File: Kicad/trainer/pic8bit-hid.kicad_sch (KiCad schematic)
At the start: 27 parts, among them K402 SYMBOL-HEADER-F-1X10, K409 HARWIN-254-F-1X16-VERTICAL, K410 LED, P401 AN1, P402 AN2

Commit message: Update
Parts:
- S403: footprint tronixio:BOURNS-PEC12R -> tronixio:BOURNS-PEC12R-SWITCH; symbol tronixio:BOURNS-PEC12R-24DENTS -> tronixio:BOURNS-PEC12R-24DENTS-SWITCH-15MM
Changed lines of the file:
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@@
     (pin "1")
   )
-  (symbol (lib_id "tronixio:BOURNS-PEC12R-24DENTS") (at 104.14 96.52 0) (unit 1)
+  (symbol (lib_id "tronixio:BOURNS-PEC12R-24DENTS-SWITCH-15MM") (at 104.14 96.52 0) (unit 1)
     (in_bom yes) (on_board yes)
     (property "Reference" "S403" (id 0) (at 104.14 87.63 0)
@@
       (effects (font (size 1.15 1.15)) hide)
     )
-    (property "Footprint" "tronixio:BOURNS-PEC12R" (id 2) (at 104.14 111.76 0)
+    (property "Footprint" "tronixio:BOURNS-PEC12R-SWITCH" (id 2) (at 104.14 111.76 0)
       (effects (font (size 1 1)) hide)
     )

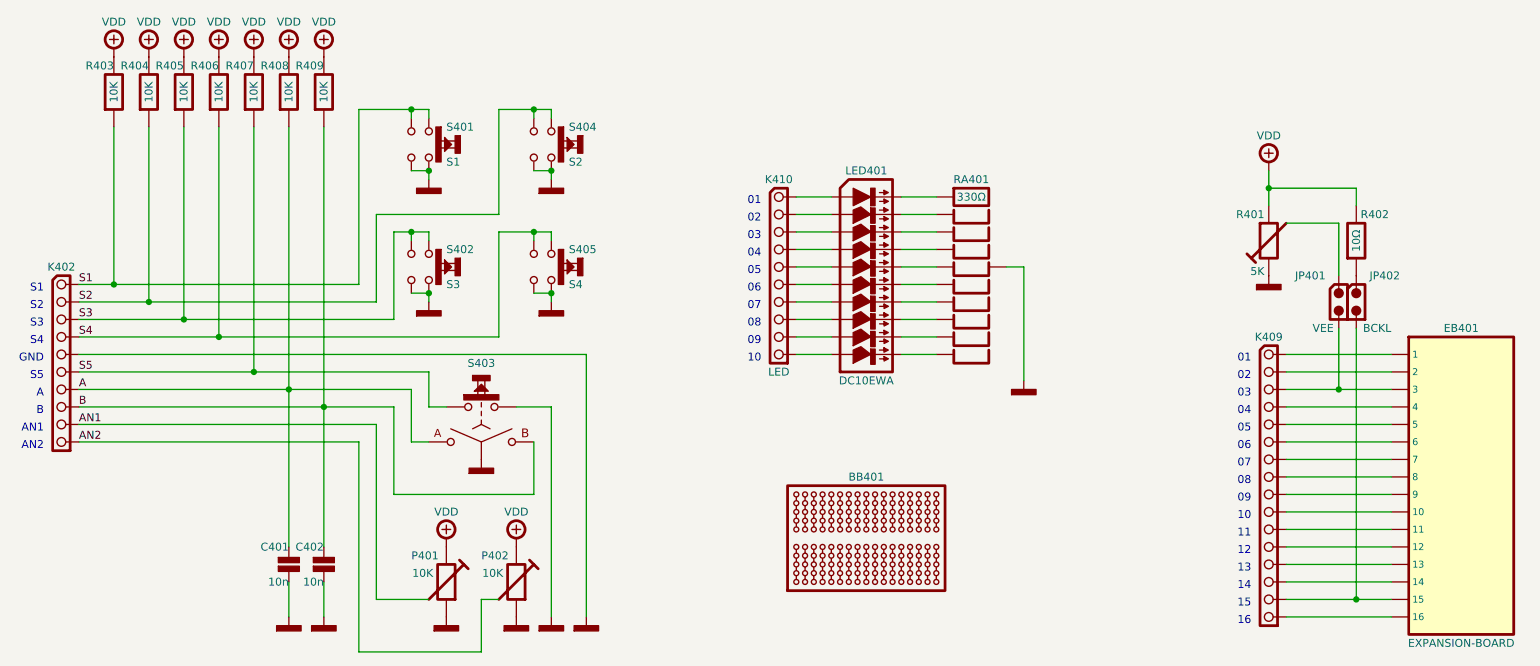
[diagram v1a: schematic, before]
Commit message: Up
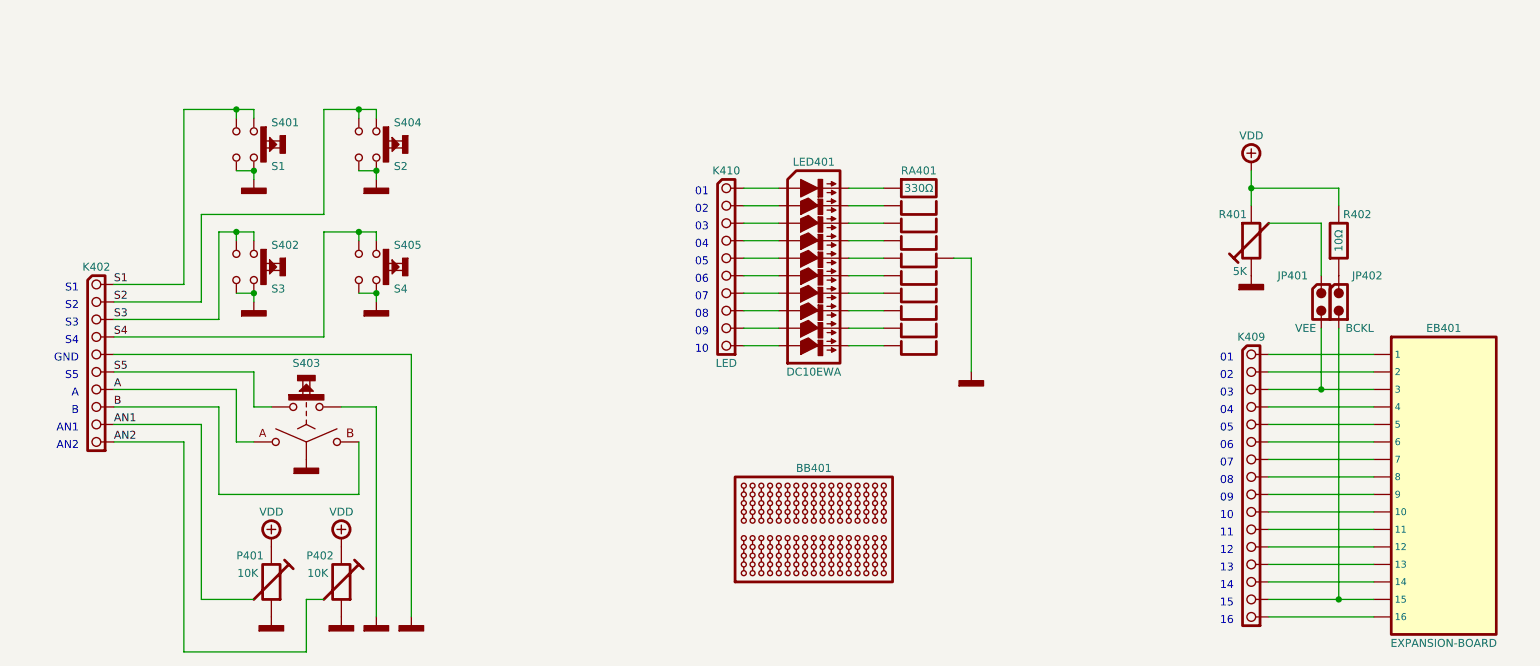
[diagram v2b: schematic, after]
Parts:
- removed C401, C402: 10n, tronixio:zzzKEMET-C315, symbol tronixio:C-0805
- removed R403, R404, R405, R406, R407, R408, R409: 10K, tronixio:RESISTOR-1016-TH, symbol tronixio:R-0805
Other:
- moved on the sheet: BB401, EB401, JP401, JP402, K402, K409, K410, LED401, P401, P402, R401, R402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
